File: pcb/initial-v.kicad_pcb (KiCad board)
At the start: 2 copper layers, 28.9 x 59.5 mm, 30 parts, among them J1 USB_C_Receptacle_USB2.0, J2 Barrel_Jack_Switch_Pin3Ring, J3 Conn_01x10, Q1 MBT3904DW1, SW1 SW_SPST, SW2 SW_SPST, U1 MCP2221AxSL, U2 MCP1700-1202E_SOT89, U3 ESP32-MINI-1-H4, U4 MPM3610GQV-Z, U5 SN65HVD230

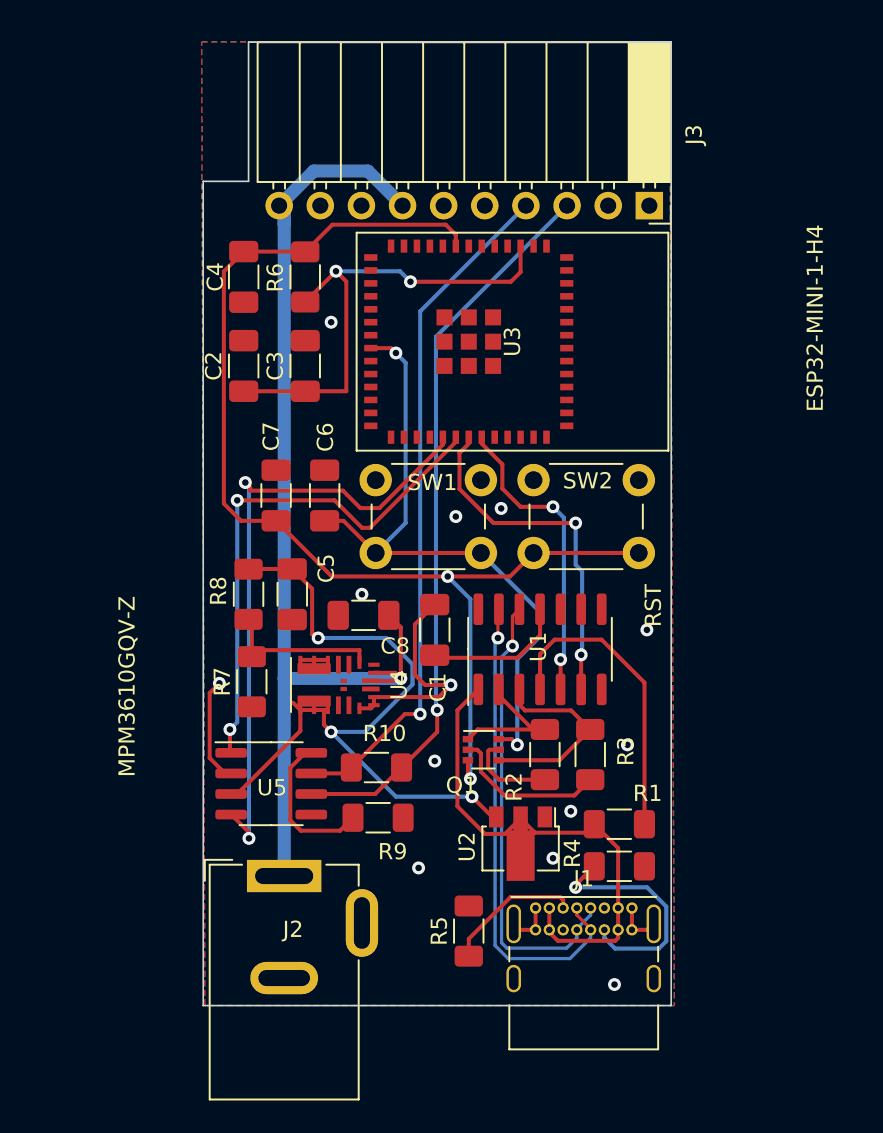
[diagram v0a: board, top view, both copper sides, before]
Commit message: updating design
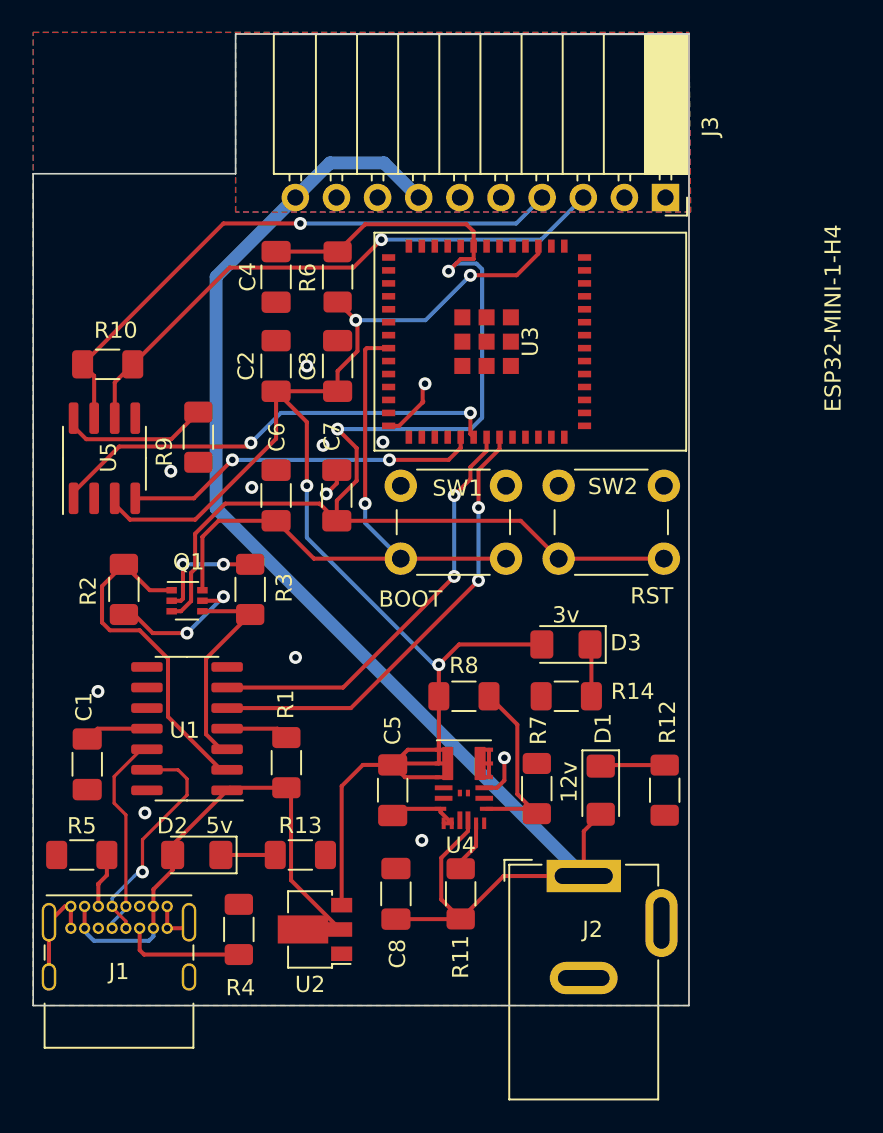
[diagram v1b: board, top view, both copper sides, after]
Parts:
- added D1: 12v, LED_SMD:LED_1206_3216Metric_Pad1.42x1.75mm_HandSolder, F.Cu at (143.6, 98.7)
- added D2: 5v, LED_SMD:LED_1206_3216Metric_Pad1.42x1.75mm_HandSolder, F.Cu at (118.6, 102.7)
- added D3: 3v, LED_SMD:LED_1206_3216Metric_Pad1.42x1.75mm_HandSolder, F.Cu at (141.4, 89.7)
- added G***: LOGO, artwork:mise, B.Cu at (112.3, 83.0)
- added R11: 100k, Resistor_SMD:R_1206_3216Metric_Pad1.30x1.75mm_HandSolder, F.Cu at (134.9, 105.1)
- added R12: 1k, Resistor_SMD:R_1206_3216Metric_Pad1.30x1.75mm_HandSolder, F.Cu at (147.5, 98.7)
- added R13: 100, Resistor_SMD:R_1206_3216Metric_Pad1.30x1.75mm_HandSolder, F.Cu at (125.0, 102.7)
- added R14: 100, Resistor_SMD:R_1206_3216Metric_Pad1.30x1.75mm_HandSolder, F.Cu at (141.4, 92.9)
- moved R10 29.9 mm to (113.1, 72.4)
- moved J1 28.7 mm to (110.8, 105.9)
- moved R2 27.9 mm to (114.1, 86.3)
- moved R9 26.0 mm to (118.7, 76.9), turned to -90 degrees
- moved R5 24.4 mm to (111.5, 102.7), turned to 180 degrees
- moved R4 23.8 mm to (121.2, 107.3), turned to 90 degrees
- moved R3 23.3 mm to (121.9, 86.3), turned to -90 degrees
- moved C1 23.0 mm to (111.8, 97.1), turned to -90 degrees
- moved U5 22.6 mm to (112.9, 78.2), turned to 90 degrees
- moved U1 22.3 mm to (118.0, 94.9), turned to 180 degrees
- moved R1 20.9 mm to (124.1, 97.0), turned to 90 degrees
- moved Q1 20.5 mm to (118.0, 87.0)
- moved R7 18.8 mm to (139.6, 98.6), turned to -90 degrees
- moved J2 18.5 mm to (142.5, 104.0)
- moved C8 17.3 mm to (130.9, 105.1), turned to 90 degrees
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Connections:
- C2 pad 1: Net-(C2-Pad1) -> +3V3
- C3 pad 1: Net-(C2-Pad1) -> +3V3
- R6 pad 1: Net-(C2-Pad1) -> +3V3
- U3 pad 3: Net-(C2-Pad1) -> +3V3
- U4 pad 17: +12V -> Net-(U4-Pad17)
- U4 pad 3: unconnected-(U4-Pad3) -> GND
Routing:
- net +3V3: track 45.1 -> 94.7 mm, vias 3 -> 4
- net Net-(C2-Pad1): track 30.2 -> 0.00 mm, vias 2 -> 0
- net +12V: track 67.3 -> 86.9 mm, vias 1 -> 0
- net /CAN_RX: track 39.0 -> 22.0 mm
- net /D-: track 28.3 -> 12.7 mm, vias 1 -> 0
- net /D+: track 29.8 -> 14.3 mm
- net Net-(R1-Pad2): track 18.8 -> 3.89 mm
- net /GP0: track 9.08 -> 21.4 mm
- net /CAN_LOW: track 45.3 -> 35.9 mm
- net /RX: track 18.9 -> 28.2 mm
- net /ESP_RST: track 73.2 -> 81.2 mm
- net Net-(J1-PadB5): track 14.8 -> 7.59 mm, vias 1 -> 0
- net /CAN_HIGH: track 42.3 -> 36.3 mm
- net Net-(J1-PadA5): track 8.53 -> 3.41 mm
- net Net-(C1-Pad1): track 8.75 -> 3.95 mm
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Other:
- board size 28.9 x 59.5 mm -> 40.5 x 60 mm
- board text added: "BOOT"
